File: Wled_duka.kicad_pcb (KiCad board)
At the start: 2 copper layers, 100 x 100 mm, 41 parts, among them J1 7775-2, J2 DATA channels, J3 CH1&2, J4 CH3&4, J5 Relay out, J6 DMX512, J7 7775-2, J8 Vin_alt, Q1 AO3400A, U1 XL1509-5.0, U2 ESP32_S3_supermini, U3 74AHCT125, U4 MAX485E

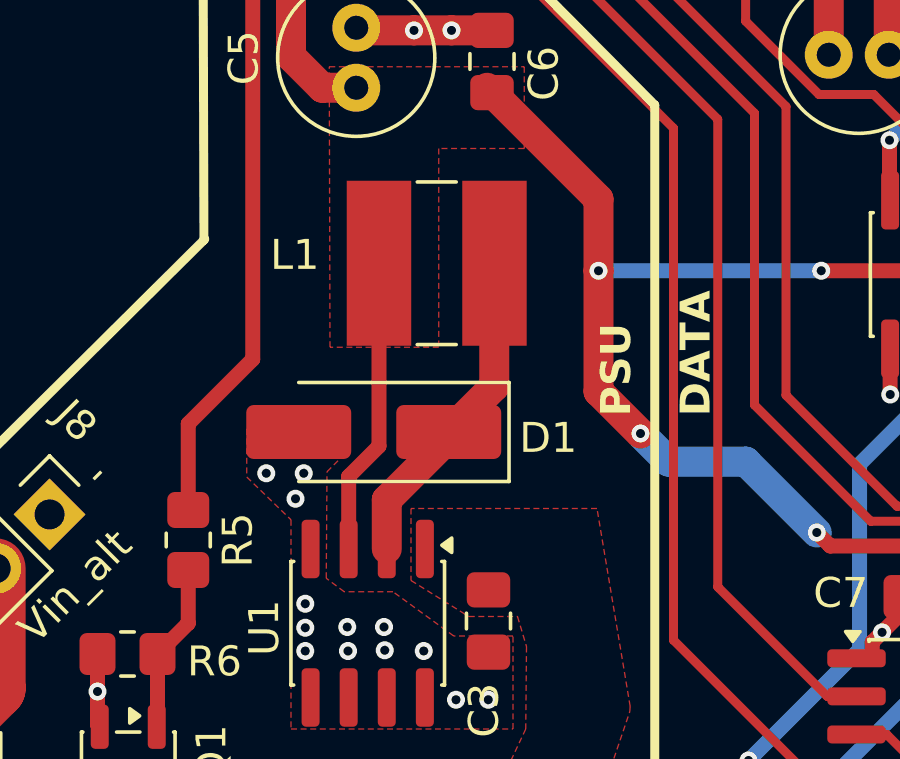
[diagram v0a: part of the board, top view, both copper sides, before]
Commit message: LDO
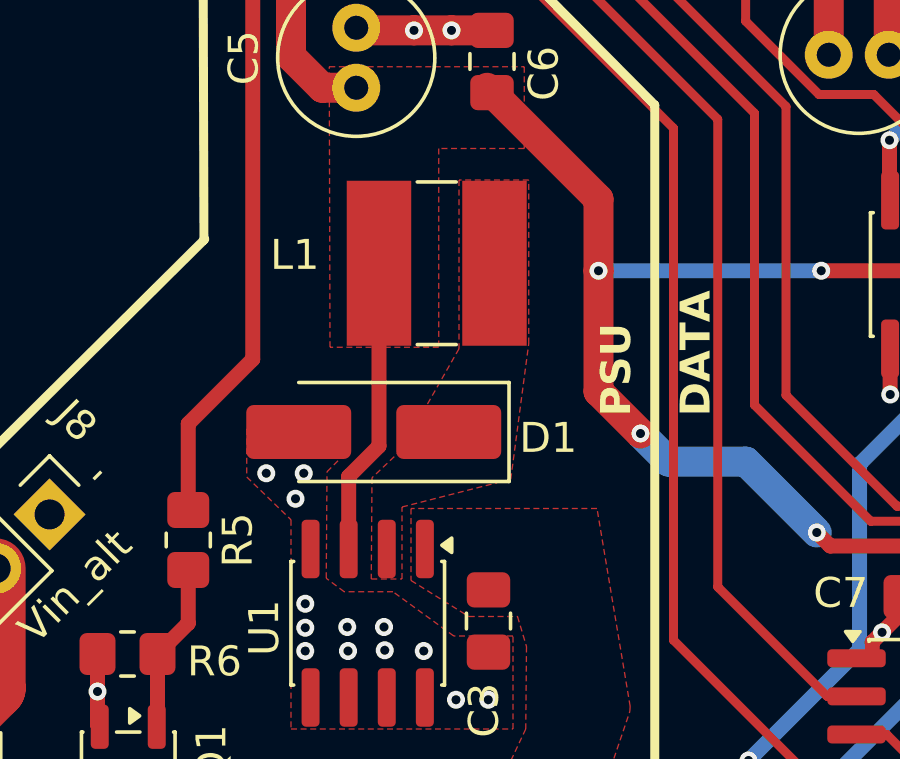
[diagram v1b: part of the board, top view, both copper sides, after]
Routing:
- net Net-(D1-K): track 11.0 -> 0.21 mm
- added copper zone on F.Cu, net Net-(D1-K)
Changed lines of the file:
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@@
-	)
-	(segment
-		(start 142.8175 124.075)
-		(end 142.8175 122.437486)
-		(width 1)
-		(layer "F.Cu")
-		(net "Net-(D1-K)")
 	)
 	(segment
@@
 	)
 	(segment
-		(start 146.4 118.6575)
-		(end 146.4 114.5575)
-		(width 1)
-		(layer "F.Cu")
-		(net "Net-(D1-K)")
-	)
-	(segment
-		(start 144.8825 120.175)
-		(end 146.4 118.6575)
-		(width 1)
-		(layer "F.Cu")
-		(net "Net-(D1-K)")
-	)
-	(segment
 		(start 144.8825 120.372486)
 		(end 144.8825 120.175)
-		(width 1)
-		(layer "F.Cu")
-		(net "Net-(D1-K)")
-	)
-	(segment
-		(start 142.8175 122.437486)
-		(end 144.8825 120.372486)
 		(width 1)
 		(layer "F.Cu")
@@
 			)
 		)
+	)
+	(zone
+		(net "Net-(D1-K)")
+		(layer "F.Cu")
+		(hatch edge 0.5)
+		(priority 4)
+		(connect_pads yes
+			(clearance 0.5)
+		)
+		(min_thickness 0.25)
+		(fill yes
+			(thermal_gap 0.5)
+			(thermal_bridge_width 0.5)
+			(smoothing fillet)
+			(radius 2)
+			(island_removal_mode 1)
+		)
+		(polygon
+			(pts
+				(xy 143.325 125.075) (xy 143.325 122.675) (xy 146.95 121.75) (xy 147.55 117.225) (xy 147.55 111.775)
+				(xy 145.225 111.775) (xy 145.225 117.4) (xy 143.3 120.775) (xy 142.325 121.7) (xy 142.3 125.075)
+			)
+		)
